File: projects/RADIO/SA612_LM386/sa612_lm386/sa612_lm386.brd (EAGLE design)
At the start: 75 x 45 mm, 29 parts, among them IC1 SA612AN_01,112, IC2 SA612AN_01,112

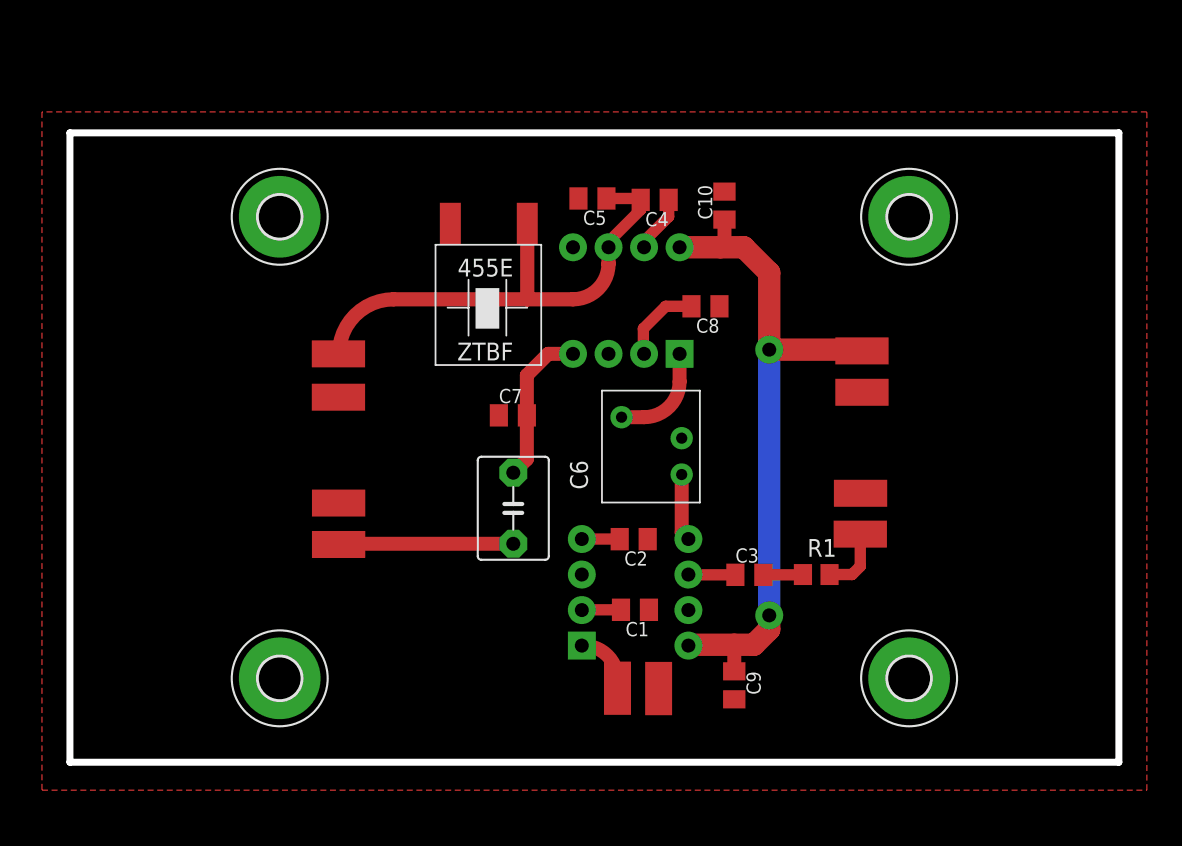
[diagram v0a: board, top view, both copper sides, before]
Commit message: update
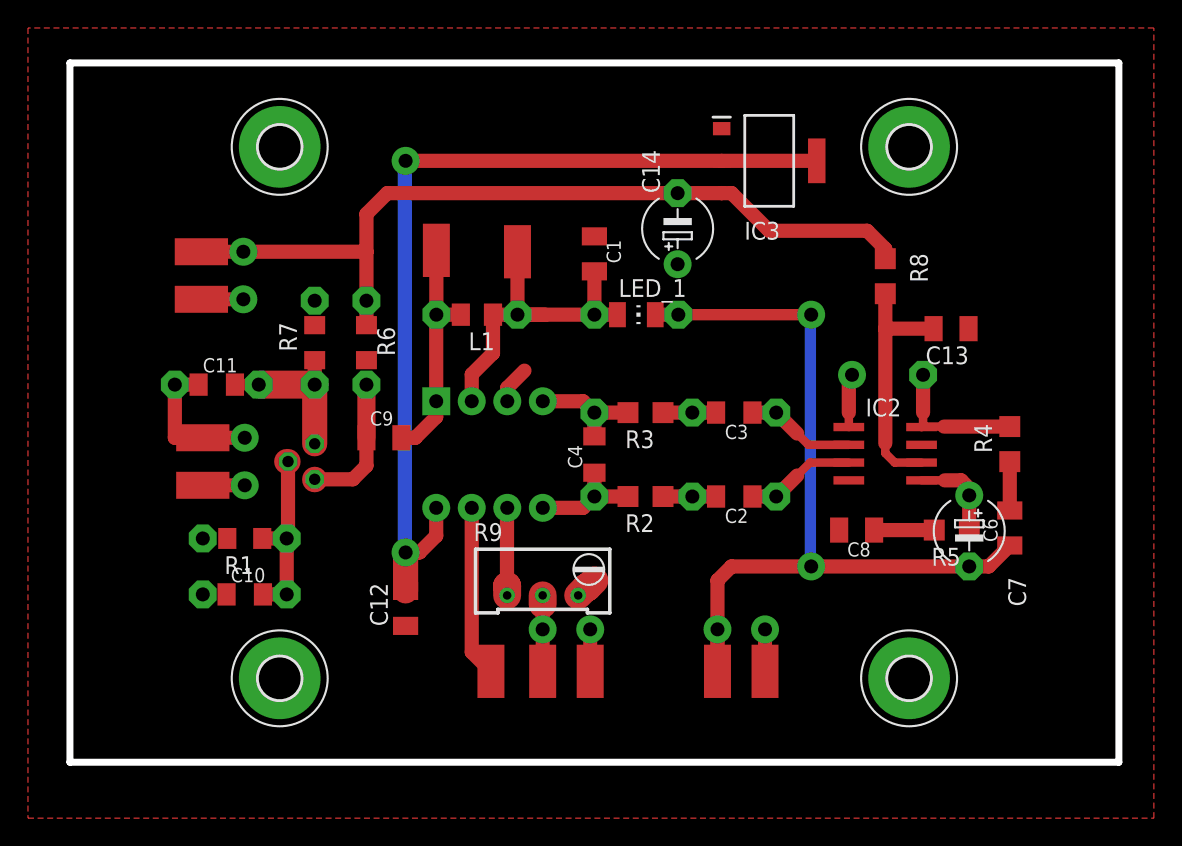
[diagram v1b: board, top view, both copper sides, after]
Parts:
- removed +5, BFI, IN, U$2, U$4, U$5, U$6, U$7, VFI: SMD_PIN, mylib:SMD_PIN
- removed U$1: ZTBF455E, mylib:ZTBF455E
- removed U$9: LT455EU, mylib:LT455EU
- added C11: 100pF, mylib:C0805K
- added C12, C13: 100nF, mylib:C0805
- added C14: 10uF, mylib:E5-5
- added CON_1, CON_2, RF_IN: 2X_SMD_PTH_PIN, mylib:2X_SMD_PTH
- added IC3: LM1117MPX-33NOPB, LM1117MPX-33NOPB:SOT230P700X180-4N
- added IN_A, IN_B, P_1: SMD_PIN, mylib:SMD_PIN
- added L1: 10uH, mylib:M0805
- added LED_1: (no value), mylib:CHIP-LED0805
- added Q1: BF245, transistor-fet:TO92
- added R2, R3: (no value), mylib:R0805W
- added R4, R5: 10k, mylib:R0805W
- added R6: (no value), mylib:R0805
- added R7: 1M, mylib:R0805
- added R8: 100, mylib:R0805W
- added R9: (no value), rcl:RTRIM64W
- C1, C8: value 10pF -> 10nF; device rcl:C0805K -> mylib:C0805
- C10: value 100nF -> 33nF; device rcl:C0805K -> mylib:C0805K
- C2, C3: value 10pF -> 20nF; device rcl:C0805K -> mylib:C0805K
- C4: value 470pF -> 33nF; device rcl:C0805K -> mylib:C0805K
- C5: value 470pF -> 10uF; device rcl:C0805K -> mylib:E5-5
- C6: value 2.2uF -> 10nF; device rcl:C050-050X075 -> mylib:C0805
- C7: value 10pF -> 47uF; device rcl:C0805K -> mylib:E5-5
- C9: value 100nF -> 10nF; device rcl:C0805K -> mylib:C0805
- IC2: value SA612AN_01,112 -> LM386M-1; device SA612AN_01_112:DIP762W53P254L950H420Q8N -> linear:SO08
- OUT: value SMD_PIN -> 2X_SMD_PTH_PIN; device mylib:SMD_PIN -> mylib:2X_SMD_PTH
- R1: value 470R -> (none); device rcl:R0805 -> mylib:R0805
- moved C10 44.2 mm to (12.5, 12.0), turned to 0 degrees
- moved R1 40.9 mm to (12.5, 16.0), turned to 180 degrees
- moved C6 35.5 mm to (67.2, 16.8), turned to 90 degrees
- moved C7 33.7 mm to (64.3, 16.5), turned to 270 degrees
- moved C9 30.7 mm to (22.4, 23.2), turned to 0 degrees
- moved OUT 30.2 mm to (48.0, 6.50)
- moved C1 25.6 mm to (37.5, 36.4), turned to 270 degrees
- moved C5 24.6 mm to (58.5, 27.7), flipped to the bottom
- moved IC2 21.5 mm to (58.3, 22.1), flipped to the top, turned to 270 degrees
- moved C8 19.3 mm to (56.2, 16.6)
- moved C4 18.7 mm to (37.5, 22.0), turned to 90 degrees
- moved IC1 14.3 mm to (30.0, 22.0), turned to 270 degrees
- moved C3 11.7 mm to (47.5, 25.0), turned to 180 degrees
- moved C2 7.81 mm to (47.5, 19.0)
- moved H3 5.00 mm to (15.0, 44.0)
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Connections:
- removed net BFI: BFI.P$1, C4.2, C5.1, IC2.6, U$1.P$1
- removed net OUT: C6.2, OUT.P$1
- removed net RF_INPUT: IC1.1, IN.P$1
- removed net VFI: R1.2, VFI.P$1
- new net 12V: C14.-, CON_2.P$1, CON_2.T$1, IC3.3, R6.1, R6.P$1, R8.1
- new net N$13: C6.2, R4.1
- new net N$14: C6.1, C7.-, LED_1.C, LED_1.CP, OUT.P$1, OUT.T$1
- new net N$15: C7.+, IC2.5, R5.1
- new net N$16: C8.1, R5.2
- new net N$17: C10.2, C10.P$2, Q1.2, R1.1, R1.P$1
- new net N$18: C9.1, Q1.1, R6.2, R6.P$2
- new net N$19: C11.2, C11.P$2, Q1.3, R7.1, R7.P$1
- new net N$2: C1.2, IC1.2, IN_B.P$1, L1.1, L1.P$1, LED_1.A, LED_1.AP
- new net N$20: C11.1, C11.P$1, RF_IN.P$1, RF_IN.T$1
- new net N$21: C13.2, IC2.6, R8.2
- new net N$22: CON_1.P$1, CON_1.T$1, R9.2
- new net N$7: C4.1, C4.P$1, IC1.5, R2.2
- new net N$9: IC1.6, R9.1
- net 5V: now also C12.2, IC3.2, IC3.4; no longer +5.P$1, C10.1, C9.1, IC2.8
- net GND: now also C10.1, C10.P$1, C12.1, C13.1, C14.+, C8.2, CON_1.P$2, CON_1.T$2, CON_2.P$2, CON_2.T$2, IC2.4, IC3.1, OUT.P$2, OUT.T$2, R1.2, R1.P$2, R7.2, R7.P$2, R9.3, RF_IN.P$2, RF_IN.T$2; no longer C10.2, C2.1, C5.2, C7.1, C8.1, C9.2, IC2.3, U$1.P$2, U$2.P$1, U$4.P$1, U$5.P$1, U$6.P$1, U$7.P$1, U$9.GND
- net N$1: now also C9.2, IC1.1, IN_A.P$1, L1.2, L1.P$2; no longer C1.2, IC1.2
- net N$10: now also IC1.7, P_1.P$1; no longer C6.1, C7.2, IC2.4
- net N$11: now also C5.+, IC2.1; no longer C8.2, IC2.2
- net N$12: now also C5.-, IC2.8, R4.2; no longer IC1.5, U$9.IN
- net N$3: now also C2.1, C2.P$1, IC2.3; no longer IC2.1, U$9.OUT
- net N$4: now also C3.1, C3.P$1, IC2.2; no longer C2.2, IC1.4
- net N$5: now also C3.P$2, R3.1; no longer R1.1
- net N$6: now also C2.2, C2.P$2, R2.1; no longer C3.1, IC1.6
- net N$8: now also C4.2, C4.P$2, IC1.4, R3.2; no longer C4.1, IC2.7
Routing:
- net N$14: track 0.00 -> 57.6 mm, vias 0 -> 2
- net 12V: track 0.00 -> 56.8 mm
- net BFI: track 35.4 -> 0.00 mm
- net N$2: track 0.00 -> 25.3 mm
- net N$21: track 0.00 -> 17.7 mm
- net 5V: track 49.6 -> 64.9 mm
- net N$1: track 2.81 -> 16.9 mm
- net N$17: track 0.00 -> 13.1 mm
- net OUT: track 12.5 -> 0.00 mm
- net N$19: track 0.00 -> 11.7 mm
- net N$18: track 0.00 -> 9.93 mm
- net N$7: track 0.00 -> 8.13 mm
- net N$20: track 0.00 -> 7.50 mm
- net N$15: track 0.00 -> 6.63 mm
- net N$9: track 0.00 -> 6.29 mm
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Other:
- board size 75 x 45 mm -> 75 x 50 mm
